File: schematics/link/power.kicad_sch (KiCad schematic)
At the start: 34 parts, among them J5 12V Alt Supply, U1 Ag9912-LP, U2 LM27762, U3 TC1262-33

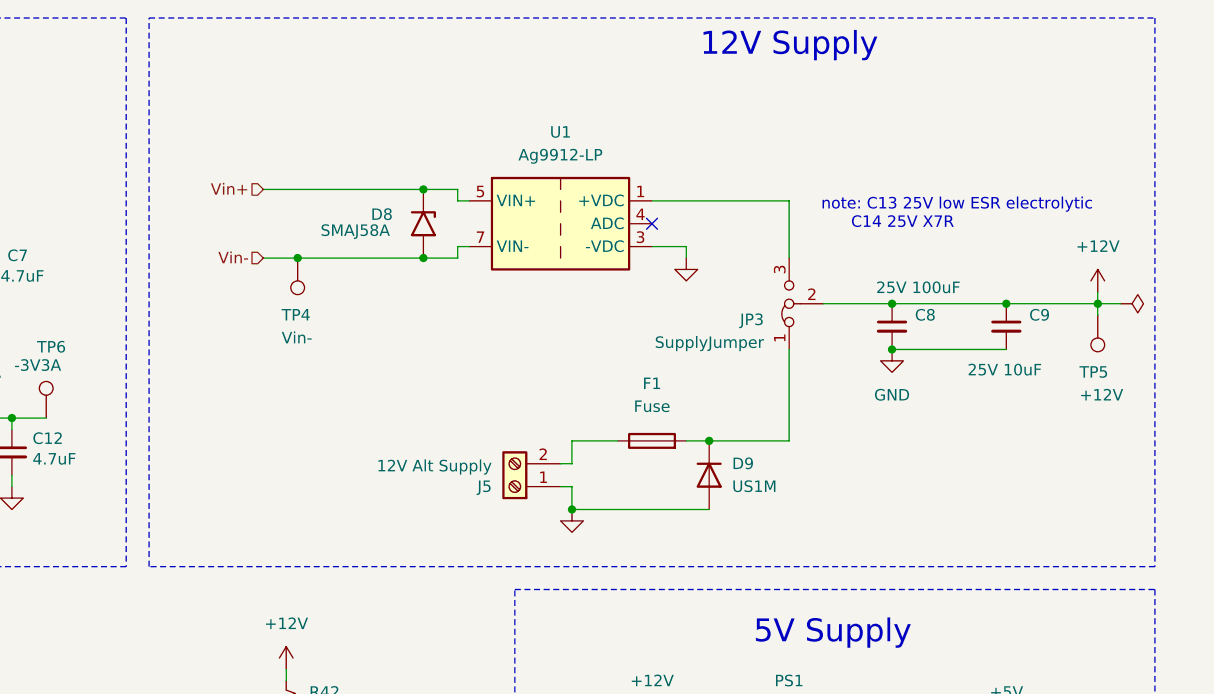
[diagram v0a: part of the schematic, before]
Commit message: fix: git history
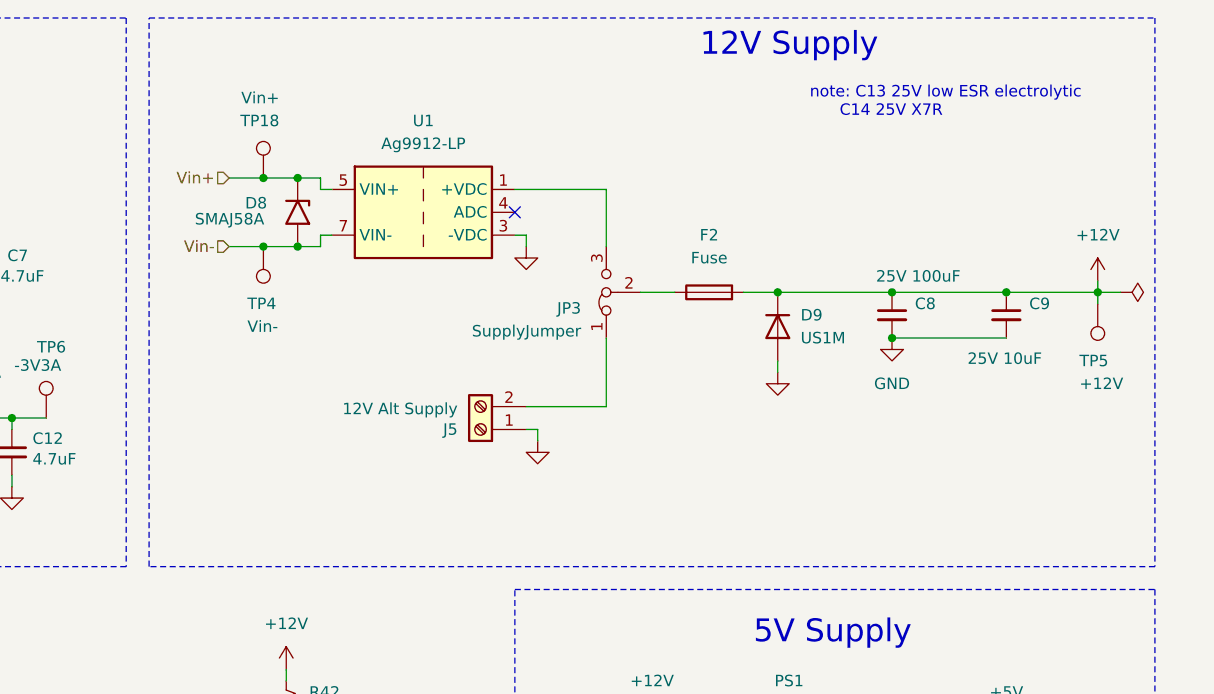
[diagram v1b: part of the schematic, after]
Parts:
- removed F1: Fuse, Link_Footprints:0154Series_LTF, symbol Device:Fuse
- added F2: Fuse, Link_Footprints:0154Series_LTF, symbol Device:Fuse
- added TP18: Vin+, Link_Footprints:TestPoint_Pad_D1.5mm, symbol Connector:TestPoint
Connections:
- net +12V: now also D9.1 (K), F2.2; no longer JP3.2 (C)
- net VIN+: now also TP18.1
- net at JP3.1 (A): now also J5.2 (Pin_2); no longer D9.1 (K)
- new net: F2.1, JP3.2 (C)
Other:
- moved on the sheet: C8, C9, D8, D9, J5, JP3, TP4, TP5, U1
